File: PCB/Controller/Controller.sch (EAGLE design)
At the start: 20 parts

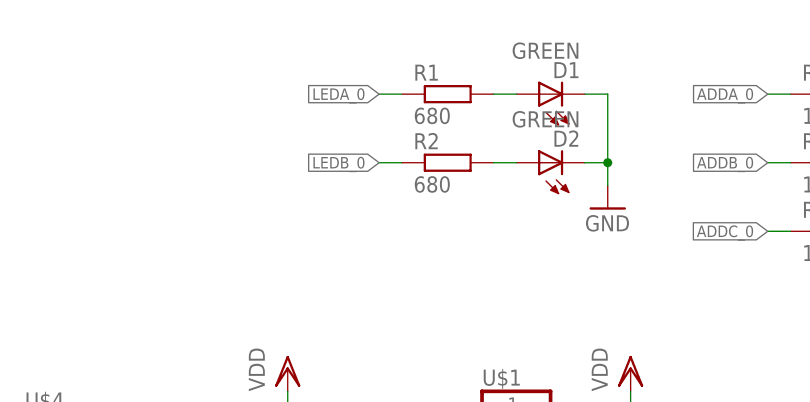
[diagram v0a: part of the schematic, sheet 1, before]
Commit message: Minor Changes
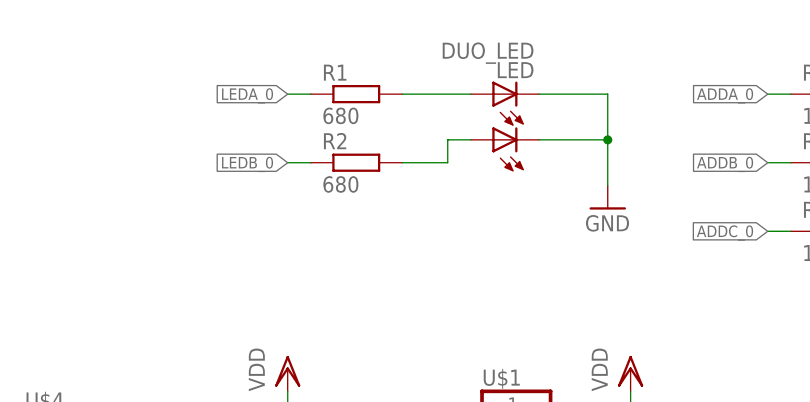
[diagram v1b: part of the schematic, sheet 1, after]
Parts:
- removed D1, D2: GREEN, led:LEDCHIP-LED0805
- added LED: DUO_LED, HeRo:DUO_LED
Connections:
- net GND: now also LED.CG, LED.CR; no longer D1.C, D2.C
- net N$1: now also LED.AG; no longer D1.A
- net N$2: now also LED.AR; no longer D2.A
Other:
- moved on the sheet: R1, R2
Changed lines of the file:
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@@
 <?xml version="1.0" encoding="utf-8"?>
 <!DOCTYPE eagle SYSTEM "eagle.dtd">
-<eagle version="9.0.0">
+<eagle version="8.7.0">
 <drawing>
 <settings>
@@
 <part name="R1" library="rcl" library_urn="urn:adsk.eagle:library:334" deviceset="R-EU_" device="R0805" package3d_urn="urn:adsk.eagle:package:23553/2" value="680"/>
 <part name="R2" library="rcl" library_urn="urn:adsk.eagle:library:334" deviceset="R-EU_" device="R0805" package3d_urn="urn:adsk.eagle:package:23553/2" value="680"/>
-<part name="D1" library="led" library_urn="urn:adsk.eagle:library:259" deviceset="LED" device="CHIP-LED0805" package3d_urn="urn:adsk.eagle:package:15818/2" value="GREEN">
-<attribute name="SPICEPREFIX" value="L"/>
-</part>
-<part name="D2" library="led" library_urn="urn:adsk.eagle:library:259" deviceset="LED" device="CHIP-LED0805" package3d_urn="urn:adsk.eagle:package:15818/2" value="GREEN">
-<attribute name="SPICEPREFIX" value="L"/>
-</part>
 <part name="GND3" library="supply1" library_urn="urn:adsk.eagle:library:371" deviceset="GND" device="">
 <attribute name="SPICEPREFIX" value="G"/>
@@
 <attribute name="SPICEPREFIX" value="G"/>
 </part>
+<part name="LED" library="HeRo" deviceset="DUO_LED" device=""/>
 </parts>
 <sheets>
@@
 <instance part="GND2" gate="1" x="43.18" y="101.6"/>
 <instance part="C1" gate="G$1" x="167.64" y="167.64"/>
-<instance part="R1" gate="G$1" x="106.68" y="170.18"/>
-<instance part="R2" gate="G$1" x="106.68" y="162.56"/>
-<instance part="D1" gate="G$1" x="116.84" y="170.18" rot="R90"/>
-<instance part="D2" gate="G$1" x="116.84" y="162.56" rot="R90"/>
+<instance part="R1" gate="G$1" x="96.52" y="170.18"/>
+<instance part="R2" gate="G$1" x="96.52" y="162.56"/>
 <instance part="GND3" gate="1" x="124.46" y="157.48"/>
 <instance part="R3" gate="G$1" x="149.86" y="170.18"/>
@@
 <instance part="R7" gate="G$1" x="193.04" y="165.1" rot="R90"/>
 <instance part="P+5" gate="1" x="193.04" y="175.26"/>
+<instance part="LED" gate="G$1" x="111.76" y="170.18" rot="R180"/>
 </instances>
 <busses>
@@
 </segment>
 <segment>
-<pinref part="D1" gate="G$1" pin="C"/>
 <pinref part="GND3" gate="1" pin="GND"/>
-<wire x1="121.92" y1="170.18" x2="124.46" y2="170.18" width="0.1524" layer="91"/>
-<wire x1="124.46" y1="170.18" x2="124.46" y2="162.56" width="0.1524" layer="91"/>
-<pinref part="D2" gate="G$1" pin="C"/>
-<wire x1="124.46" y1="162.56" x2="124.46" y2="160.02" width="0.1524" layer="91"/>
-<wire x1="121.92" y1="162.56" x2="124.46" y2="162.56" width="0.1524" layer="91"/>
-<junction x="124.46" y="162.56"/>
+<wire x1="124.46" y1="170.18" x2="124.46" y2="165.1" width="0.1524" layer="91"/>
+<wire x1="124.46" y1="165.1" x2="124.46" y2="160.02" width="0.1524" layer="91"/>
+<pinref part="LED" gate="G$1" pin="CR"/>
+<wire x1="116.84" y1="165.1" x2="124.46" y2="165.1" width="0.1524" layer="91"/>
+<junction x="124.46" y="165.1"/>
+<pinref part="LED" gate="G$1" pin="CG"/>
+<wire x1="116.84" y1="170.18" x2="124.46" y2="170.18" width="0.1524" layer="91"/>
 </segment>
 <segment>
@@
 <segment>
 <pinref part="R2" gate="G$1" pin="1"/>
-<wire x1="101.6" y1="162.56" x2="99.06" y2="162.56" width="0.1524" layer="91"/>
-<label x="99.06" y="162.56" size="1.27" layer="95" rot="R180" xref="yes"/>
+<wire x1="91.44" y1="162.56" x2="88.9" y2="162.56" width="0.1524" layer="91"/>
+<label x="88.9" y="162.56" size="1.27" layer="95" rot="R180" xref="yes"/>
 </segment>
 </net>
@@
 <segment>
 <pinref part="R1" gate="G$1" pin="1"/>
-<wire x1="101.6" y1="170.18" x2="99.06" y2="170.18" width="0.1524" layer="91"/>
-<label x="99.06" y="170.18" size="1.27" layer="95" rot="R180" xref="yes"/>
+<wire x1="91.44" y1="170.18" x2="88.9" y2="170.18" width="0.1524" layer="91"/>
+<label x="88.9" y="170.18" size="1.27" layer="95" rot="R180" xref="yes"/>
 </segment>
 </net>
@@
 <segment>
 <pinref part="R1" gate="G$1" pin="2"/>
-<pinref part="D1" gate="G$1" pin="A"/>
-<wire x1="111.76" y1="170.18" x2="114.3" y2="170.18" width="0.1524" layer="91"/>
+<pinref part="LED" gate="G$1" pin="AG"/>
+<wire x1="101.6" y1="170.18" x2="109.22" y2="170.18" width="0.1524" layer="91"/>
 </segment>
 </net>
@@
 <segment>
 <pinref part="R2" gate="G$1" pin="2"/>
-<pinref part="D2" gate="G$1" pin="A"/>
-<wire x1="111.76" y1="162.56" x2="114.3" y2="162.56" width="0.1524" layer="91"/>
-</segment>
-</net>
+<wire x1="101.6" y1="162.56" x2="106.68" y2="162.56" width="0.1524" layer="91"/>
+<wire x1="106.68" y1="162.56" x2="106.68" y2="165.1" width="0.1524" layer="91"/>
+<pinref part="LED" gate="G$1" pin="AR"/>
+<wire x1="106.68" y1="165.1" x2="109.22" y2="165.1" width="0.1524" layer="91"/>
+</segment>
+</net>

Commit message: finalised routing, added 3D-Models
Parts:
- LEG_0: value ATTINY1614 -> ATTINY16142; device HeRo:ATTINY1614 -> HeRo:ATTINY16142
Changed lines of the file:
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@@
 <?xml version="1.0" encoding="utf-8"?>
 <!DOCTYPE eagle SYSTEM "eagle.dtd">
-<eagle version="8.7.0">
+<eagle version="9.1.1">
 <drawing>
 <settings>
@@
 <part name="FRAME1" library="frames" library_urn="urn:adsk.eagle:library:229" deviceset="DINA4_L" device=""/>
 <part name="FRAME2" library="frames" library_urn="urn:adsk.eagle:library:229" deviceset="DINA4_L" device=""/>
-<part name="LEG_0" library="HeRo" deviceset="ATTINY1614" device="">
+<part name="LEG_0" library="HeRo" library_urn="urn:adsk.eagle:library:4344731" deviceset="ATTINY1614" device="2" package3d_urn="urn:adsk.eagle:package:4344597/1" value="ATTINY16142">
 <attribute name="SPICEPREFIX" value="X"/>
 </part>
@@
 <attribute name="SPICEPREFIX" value="G"/>
 </part>
-<part name="U$1" library="HeRo" deviceset="SERVO" device=""/>
-<part name="U$2" library="HeRo" deviceset="SERVO" device=""/>
-<part name="U$3" library="HeRo" deviceset="SERVO" device=""/>
+<part name="U$1" library="HeRo" library_urn="urn:adsk.eagle:library:4344731" deviceset="SERVO" device="" package3d_urn="urn:adsk.eagle:package:4344791/2"/>
+<part name="U$2" library="HeRo" library_urn="urn:adsk.eagle:library:4344731" deviceset="SERVO" device="" package3d_urn="urn:adsk.eagle:package:4344791/2"/>
+<part name="U$3" library="HeRo" library_urn="urn:adsk.eagle:library:4344731" deviceset="SERVO" device="" package3d_urn="urn:adsk.eagle:package:4344791/2"/>
 <part name="P+2" library="supply1" library_urn="urn:adsk.eagle:library:371" deviceset="+5V" device="">
 <attribute name="SPICEPREFIX" value="G"/>
@@
 <attribute name="SPICEPREFIX" value="G"/>
 </part>
-<part name="U$4" library="HeRo" deviceset="PINHEAD10SMD" device=""/>
-<part name="U$5" library="HeRo" deviceset="PINHEAD2SMD" device=""/>
-<part name="U$6" library="HeRo" deviceset="SERVO" device=""/>
-<part name="U$7" library="HeRo" deviceset="SERVO" device=""/>
-<part name="U$8" library="HeRo" deviceset="SERVO" device=""/>
+<part name="U$4" library="HeRo" library_urn="urn:adsk.eagle:library:4344731" deviceset="PINHEAD10SMD" device="" package3d_urn="urn:adsk.eagle:package:4344790/2"/>
+<part name="U$5" library="HeRo" library_urn="urn:adsk.eagle:library:4344731" deviceset="PINHEAD2SMD" device="" package3d_urn="urn:adsk.eagle:package:4344788/2"/>
+<part name="U$6" library="HeRo" library_urn="urn:adsk.eagle:library:4344731" deviceset="SERVO" device="" package3d_urn="urn:adsk.eagle:package:4344791/2"/>
+<part name="U$7" library="HeRo" library_urn="urn:adsk.eagle:library:4344731" deviceset="SERVO" device="" package3d_urn="urn:adsk.eagle:package:4344791/2"/>
+<part name="U$8" library="HeRo" library_urn="urn:adsk.eagle:library:4344731" deviceset="SERVO" device="" package3d_urn="urn:adsk.eagle:package:4344791/2"/>
 <part name="VDD3" library="supply1" library_urn="urn:adsk.eagle:library:371" deviceset="VDD" device="">
 <attribute name="SPICEPREFIX" value="G"/>
@@
 <attribute name="SPICEPREFIX" value="G"/>
 </part>
-<part name="LED" library="HeRo" deviceset="DUO_LED" device=""/>
+<part name="LED" library="HeRo" library_urn="urn:adsk.eagle:library:4344731" deviceset="DUO_LED" device="" package3d_urn="urn:adsk.eagle:package:4344780/2"/>
 </parts>
 <sheets>
